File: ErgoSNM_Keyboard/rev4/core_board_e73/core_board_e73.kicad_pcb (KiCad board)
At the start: 2 copper layers, 68.5 x 53 mm, 58 parts, among them J1 USB_C_Receptacle_USB2.0, J2 Conn_02x10_Odd_Even, J3 Conn_02x10_Odd_Even, J4 PJ-393_TRRS_8P, J5 PJ-393_TRRS_8P, J6 Conn_Batt, J7 Debug, J8 Conn_02x05_Odd_Even, J9 Conn_02x05_Odd_Even, SW1 SW_SPDT, SW2 SW_SPDT, U1 E73-2G4M08S1C, U2 USBLC6-2SC6, U3 BQ24075RGT, U4 TPS63900, Y1 32.768kHz

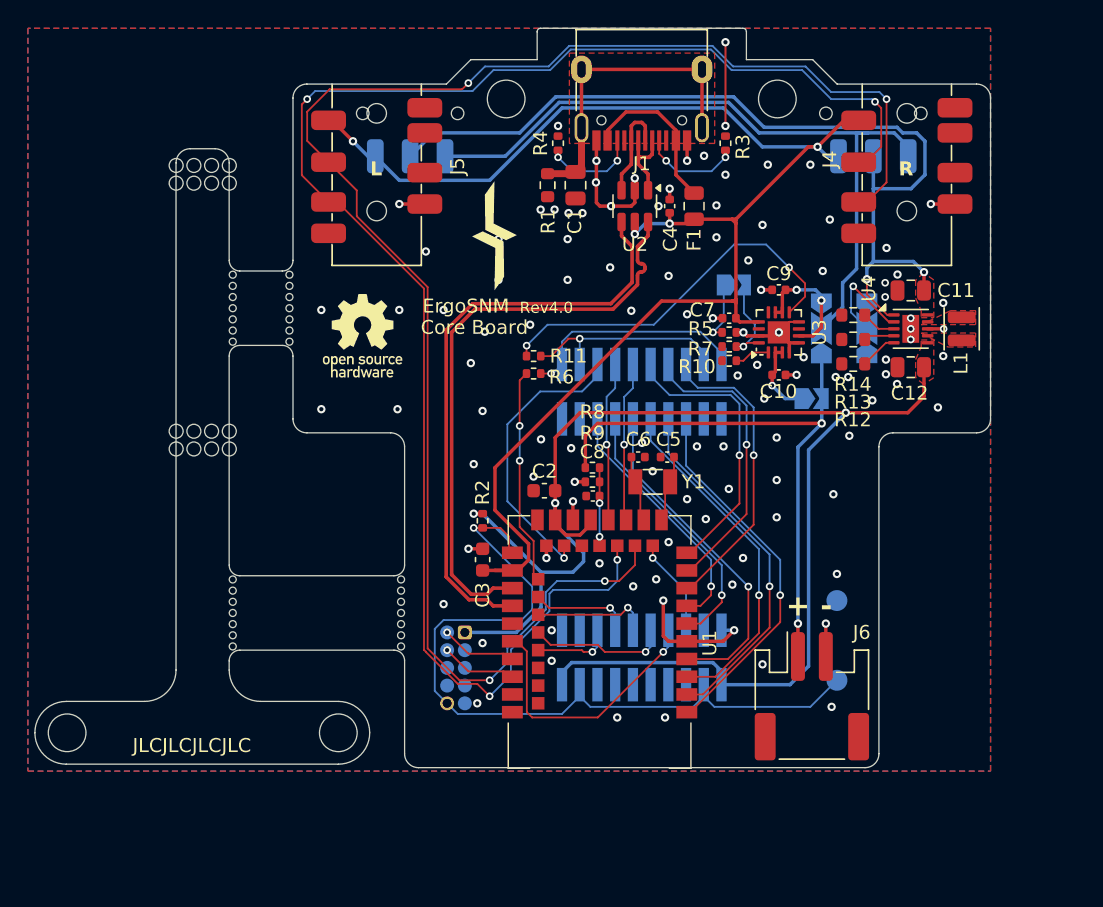
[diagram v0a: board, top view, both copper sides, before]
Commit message: feat: update E73 core board
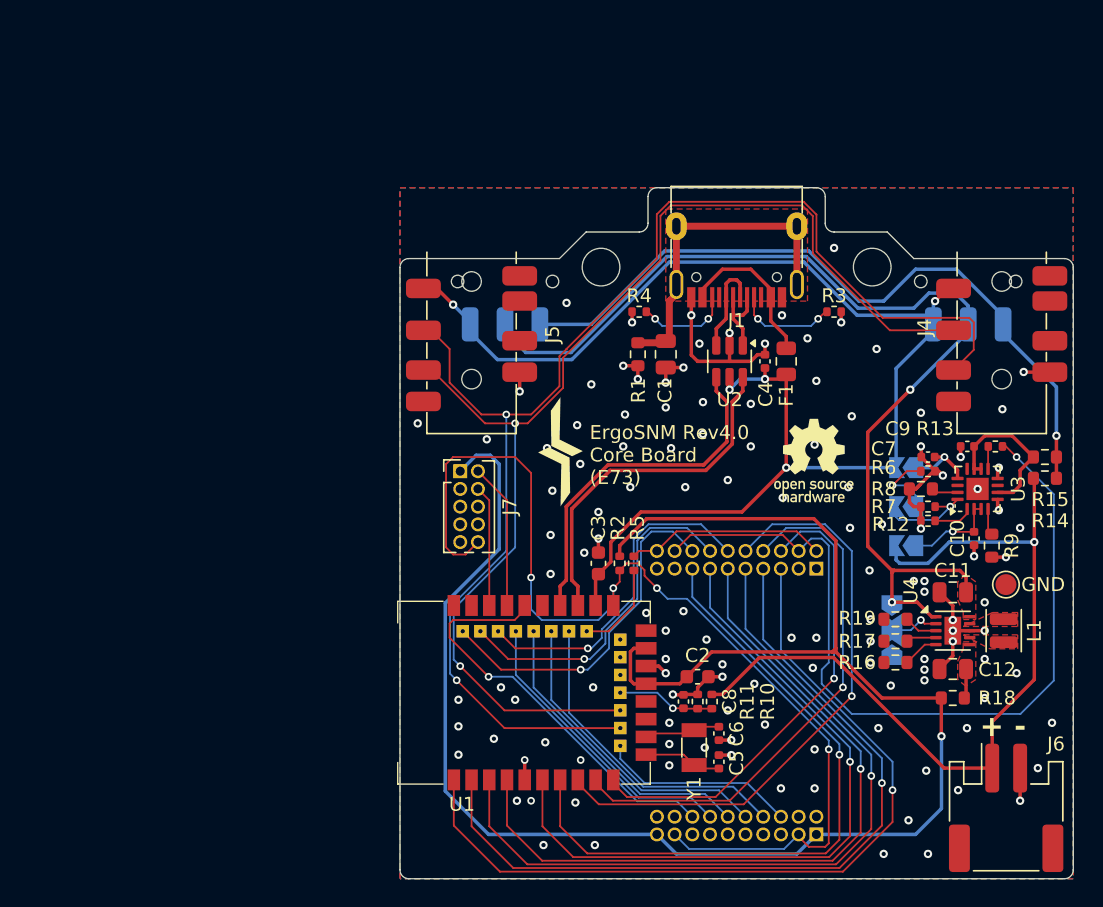
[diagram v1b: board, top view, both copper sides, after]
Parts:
- removed H23, H5, H6, H7: MountingHole, ErgoSNM_Keyboard:mouse_bit
- removed H3, H4: MountingHole, MountingHole:MountingHole_2.7mm_M2.5_ISO7380
- removed J8, J9: Conn_02x05_Odd_Even, Connector_PinHeader_1.27mm:PinHeader_2x04_P1.27mm_Vertical
- removed the SB3 at (154.1, 92.6)
- removed the TP1 at (155.2, 117.8)
- added R14: 0R, Resistor_SMD:R_0603_1608Metric, F.Cu at (170.1, 103.3)
- added R15: 0R, Resistor_SMD:R_0603_1608Metric, F.Cu at (170.1, 101.8)
- added R18: 0R, Resistor_SMD:R_0603_1608Metric, F.Cu at (163.5, 119.1)
- added R8: 0R, Resistor_SMD:R_0603_1608Metric, F.Cu at (161.2, 104.1)
- added R9: 0R, Resistor_SMD:R_0603_1608Metric, F.Cu at (166.3, 108.2)
- added SB2: LiPo_CHG, Jumper:SolderJumper-2_P1.3mm_Open_TrianglePad1.0x1.5mm, B.Cu at (160.2, 102.6)
- J2, J3: footprint Connector_PinHeader_1.27mm:PinHeader_2x10_P1.27mm_Vertical_SMD -> Connector_PinHeader_1.27mm:PinHeader_2x10_P1.27mm_Vertical
- J7: footprint ErgoSNM_Keyboard:SWD 10pin -> Connector_PinHeader_1.27mm:PinHeader_2x05_P1.27mm_Vertical; moved to F.Cu
- R16: renamed from R12; value 1.2k 1% -> 15k 1%
- R19: renamed from R14; value 30k 1% -> 20k 1%
- SB3: renamed from SB2; value LiPo_CHG -> LiPo_BATT
- TP1: renamed from TP2; moved to F.Cu
- U1: footprint ErgoSNM_Keyboard:E73-2G4M08S1C-52840_PCBA -> ErgoSNM_Keyboard:E73-2G4M08S1C-52840_Hand
- moved R13 33.7 mm to (166.5, 101.1)
- moved C5 22.2 mm to (146.7, 123.7), turned to -90 degrees
- moved R19 22.0 mm to (159.4, 113.5)
- moved C11 21.8 mm to (163.5, 111.5)
- moved C12 21.8 mm to (163.5, 117.0)
- moved L1 21.8 mm to (167.1, 114.3)
- moved U4 21.8 mm to (163.5, 114.3)
- moved R17 21.8 mm to (159.4, 115.0)
- moved SB4 21.7 mm to (159.1, 114.2)
- moved R16 21.6 mm to (159.4, 116.5)
- moved C6 20.6 mm to (146.7, 121.6), turned to 90 degrees
- moved SB1 20.1 mm to (160.2, 105.4), turned to 180 degrees
- moved Y1 19.3 mm to (145.0, 122.7), turned to 90 degrees
- moved R10 18.8 mm to (146.2, 119.3), turned to -90 degrees
- moved R12 18.3 mm to (161.7, 106.4)
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- renumbered R8 to R10, R9 to R11, R10 to R12, R11 to R13, R13 to R17, R6 to R5, R5 to R6
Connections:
- net /CONN_D+ renamed /power/CONN_D+
- net /CONN_D- renamed /power/CONN_D-
- net /OUT_SEL renamed /power/OUT_SEL
- net /USB_SH renamed /power/USB_SH
- net /VBATT_SRC renamed /power/VBATT_SRC
- net /VIN_DCDC renamed /power/VIN_DCDC
- C12 pad 1: VDD -> /power/VOUT_DCDC
- C7 pad 1: VBUS -> Net-(SB2-A)
- U1 pad 10: COL_IO_2 -> COL_IO_0
- U1 pad 15: COL_IO_3 -> unconnected-(U1-P0.05-Pad15)
- U1 pad 17: COL_IO_4 -> unconnected-(U1-P1.09-Pad17)
- U1 pad 22: COL_IO_5 -> unconnected-(U1-P0.07-Pad22)
- U1 pad 30: HS_IO_4 -> HS_IO_1
- U1 pad 32: HS_IO_3 -> HS_IO_2
- U1 pad 34: HS_IO_2 -> HS_IO_3
- U1 pad 35: HS_IO_1 -> HS_IO_5
- U1 pad 36: HS_IO_5 -> HS_IO_4
- U1 pad 38: unconnected-(U1-P1.02-Pad38) -> COL_IO_3
- U1 pad 40: unconnected-(U1-P1.04-Pad40) -> COL_IO_4
- U1 pad 42: unconnected-(U1-P1.06-Pad42) -> COL_IO_5
- U1 pad 8: COL_IO_0 -> COL_IO_2
- U3 pad 13: VBUS -> Net-(SB2-A)
- U3 pad 15: GND -> Net-(U3-SYSOFF)
- U3 pad 4: GND -> Net-(U3-~{CE})
- U4 pad 6: VDD -> /power/VOUT_DCDC
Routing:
- net CHG_LED: track 15.3 -> 59.7 mm
- net ROW_IO_0: track 26.5 -> 58.8 mm
- net ROW_IO_1: track 25.6 -> 56.9 mm
- net ROW_IO_4: track 19.2 -> 50.0 mm
- net ROW_IO_5: track 17.8 -> 48.1 mm
- net ROW_IO_2: track 24.8 -> 55.0 mm
- net ROW_IO_3: track 23.9 -> 53.1 mm
- net RX: track 115.8 -> 86.7 mm, vias 4 -> 2
- net Net-(U3-~{CHG}): track 27.4 -> 1.62 mm, vias 2 -> 0
- net VDD: track 103.9 -> 129.5 mm, vias 3 -> 1
- net HS_IO_5: track 5.64 -> 30.1 mm
- net COL_IO_2: track 20.2 -> 43.1 mm
- net TX: track 117.6 -> 96.0 mm, vias 4 -> 2
- net RESET: track 57.0 -> 76.3 mm, vias 1 -> 4
- net COL_IO_1: track 20.8 -> 38.5 mm
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- added copper zone on F.Cu, net /power/VOUT_DCDC
- removed copper zone on F.Cu, net VDD
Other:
- board size 68.5 x 53 mm -> 48.3 x 49.5 mm
- board text added: "BAT"
- board text added: "ErgoSNM Rev4.0 Core Board (E73)"
- board text added: "USB"
- board text removed: "CHG"
- board text removed: "Core Board"
- board text removed: "ErgoSNM"
- board text removed: "L"
- board text removed: "OFF"
- board text removed: "ON"
- board text removed: "R"
- board text removed: "Rev${REVISION}"
- board text removed: "STA"
- board text removed: "Unit: mm"
